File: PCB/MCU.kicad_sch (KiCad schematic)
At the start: 29 parts, among them J1 SWD, SW65 USB Boot, SW66 Reset, U2 W25Q128JVS, U3 RP2040, U7 74LVC1T45, Y1 12MHz

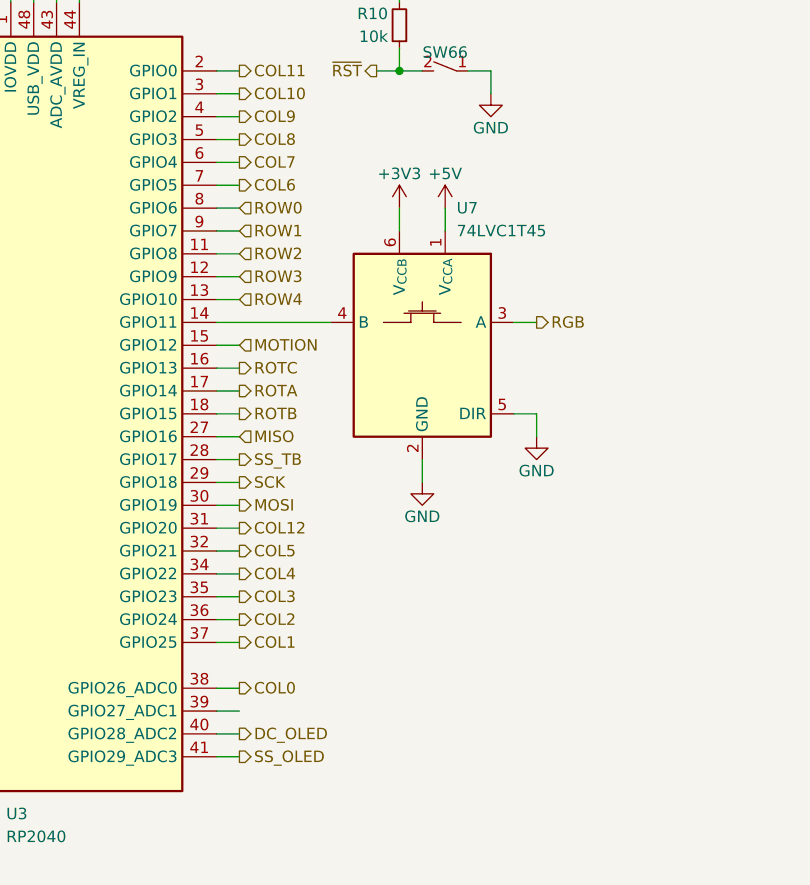
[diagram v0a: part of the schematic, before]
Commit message: Initial V2.0 update.
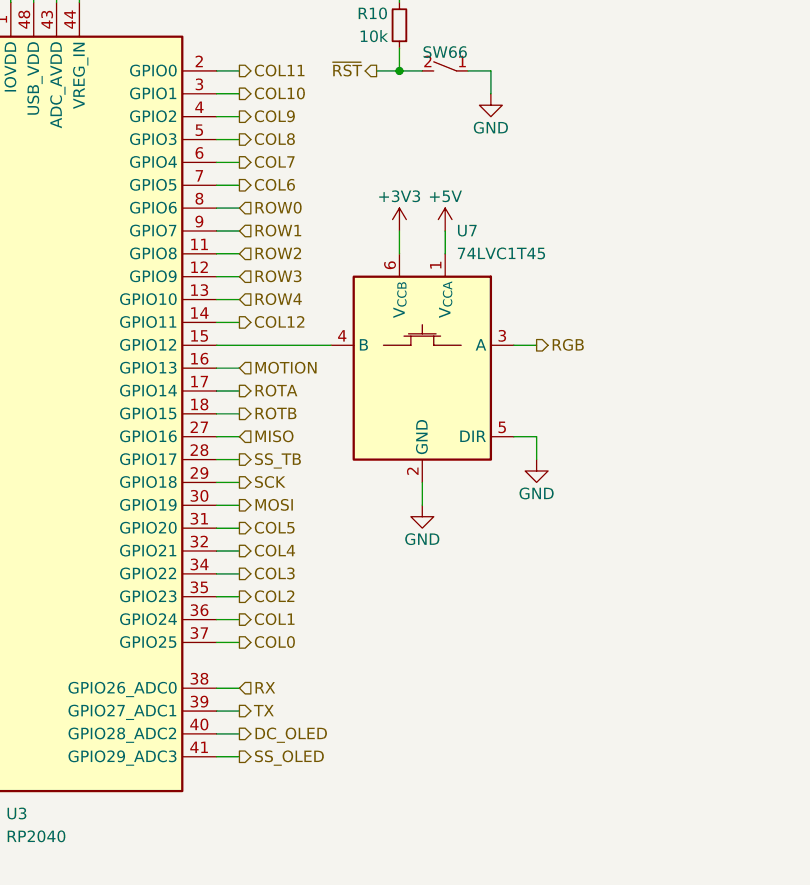
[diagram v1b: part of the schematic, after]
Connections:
- net ROTC is gone; now on net MOTION: U3.16 (GPIO13)
- net COL0: now also U3.37 (GPIO25); no longer U3.38 (GPIO26_ADC0)
- net COL1: now also U3.36 (GPIO24); no longer U3.37 (GPIO25)
- net COL12: now also U3.14 (GPIO11); no longer U3.31 (GPIO20)
- net COL2: now also U3.35 (GPIO23); no longer U3.36 (GPIO24)
- net COL3: now also U3.34 (GPIO22); no longer U3.35 (GPIO23)
- net COL4: now also U3.32 (GPIO21); no longer U3.34 (GPIO22)
- net COL5: now also U3.31 (GPIO20); no longer U3.32 (GPIO21)
- net MOTION: no longer U3.15 (GPIO12)
- net at U7.4 (B): now also U3.15 (GPIO12); no longer U3.14 (GPIO11)
- net TX: now reaches U3.39 (GPIO27_ADC1)
- new net RX: U3.38 (GPIO26_ADC0)
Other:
- moved on the sheet: U7

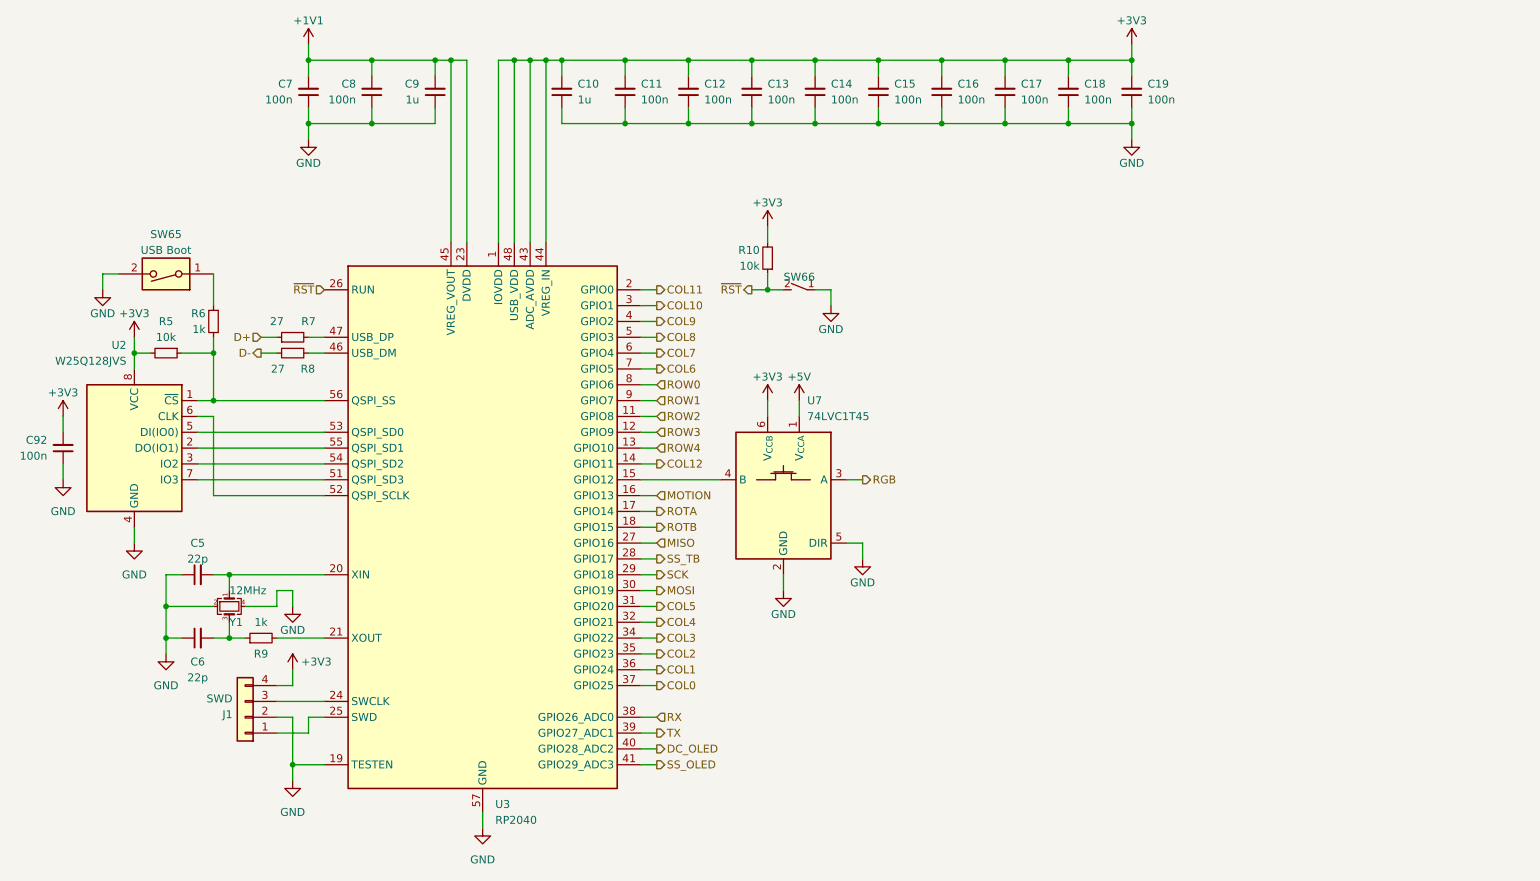
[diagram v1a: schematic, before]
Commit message: Additional changes.
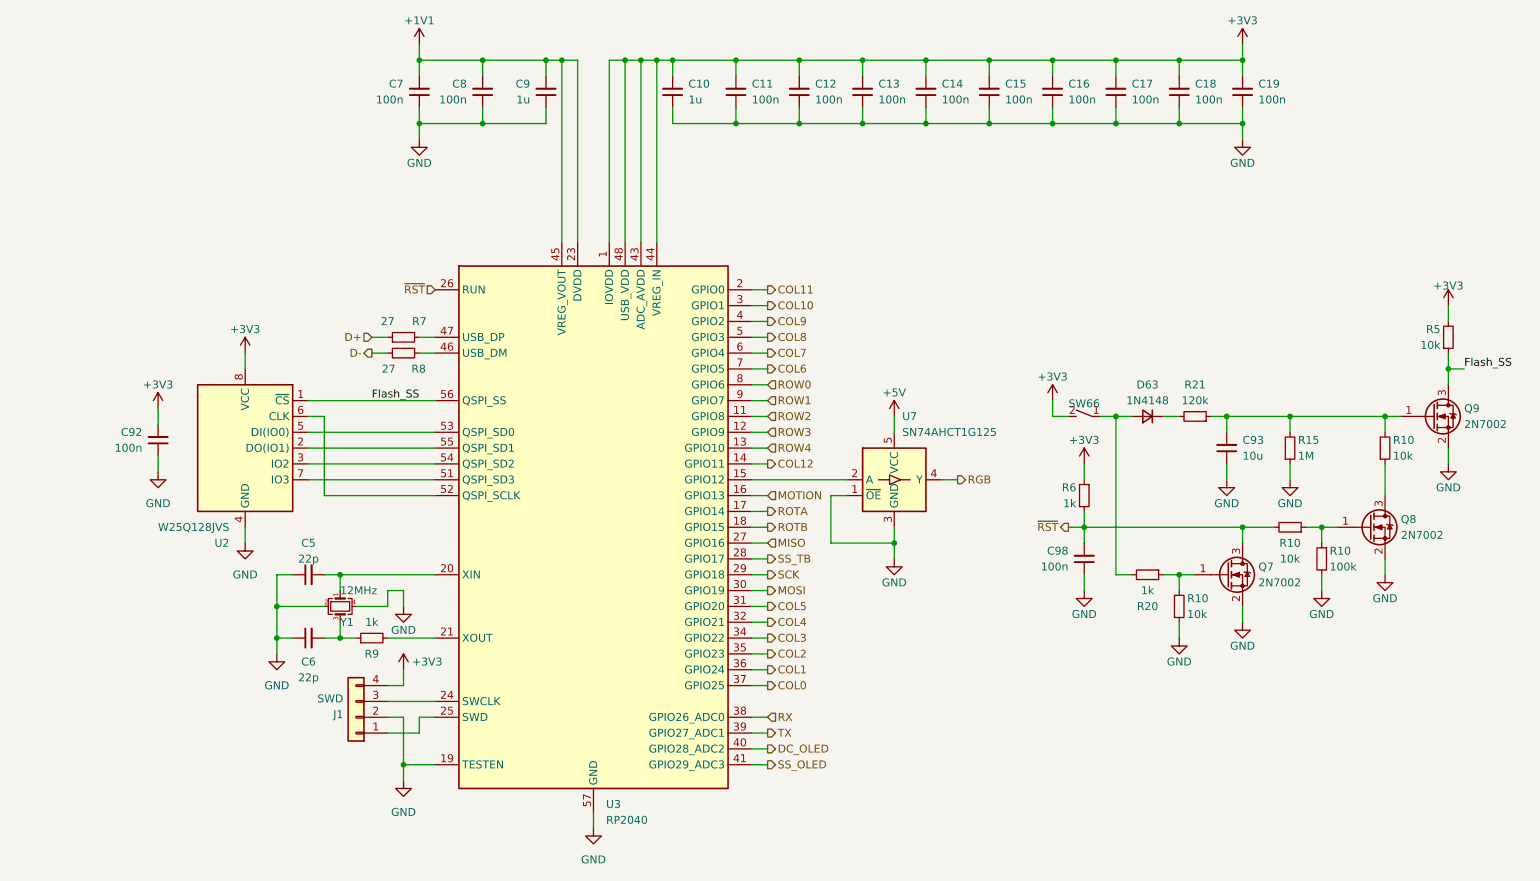
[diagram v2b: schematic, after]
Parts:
- removed R10: 10k, Resistor_SMD:R_0402_1005Metric, symbol Device:R_Small
- removed SW65: USB Boot, Button_Switch_SMD:SW_DIP_SPSTx01_Slide_6.7x4.1mm_W8.61mm_P2.54mm_LowProfile, symbol Switch:SW_DIP_x01
- removed U7: 74LVC1T45, Package_TO_SOT_SMD:SOT-363_SC-70-6, symbol Cantaloupe:74LVC1T45
- added C93: 10u, Capacitor_SMD:C_0603_1608Metric, symbol Device:C_Small
- added C98: 100n, Capacitor_SMD:C_0402_1005Metric, symbol Device:C_Small
- added D63: 1N4148, Honeydew:D_SOD-323, symbol Device:D_Small
- added Q7, Q8, Q9: 2N7002, Package_TO_SOT_SMD:SOT-23, symbol Transistor_FET:2N7002
- added R10: 100k, Resistor_SMD:R_0402_1005Metric, symbol Device:R_Small
- added R10 (x3): 10k, Resistor_SMD:R_0402_1005Metric, symbol Device:R_Small
- added R15: 1M, Resistor_SMD:R_0402_1005Metric, symbol Device:R_Small
- added R20: 1k, Resistor_SMD:R_0402_1005Metric, symbol Device:R_Small
- added R21: 120k, Resistor_SMD:R_0402_1005Metric, symbol Device:R_Small
- added U7: SN74AHCT1G125, Package_TO_SOT_SMD:SOT-23-5, symbol Honeydew:SN74AHCT1G125
- R5: now in the parts list
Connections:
- net +3V3: now also R6.1, SW66.2 (B)
- net +5V: now also U7.5 (VCC)
- net GND: now also C93.1, C98.1, Q7.2 (S), Q8.2 (S), Q9.2 (S), R10.1, R10.2, R15.1, U7.1 (~{OE}), U7.3 (GND); no longer SW66.1 (A)
- net RGB: now also U7.4 (Y)
- net ~{RST}: now also R6.2, C98.2, Q7.3 (D), R10.2; no longer SW66.2 (B)
- net Flash_SS: now reaches R5.1, U2.1 (~{CS}), U3.56 (QSPI_SS)
- net Flash_SS: now also Q9.3 (D); no longer R6.2
- net at U3.15 (GPIO12): now also U7.2 (A)
- new net: Q7.1 (G), R10.2, R20.1
- new net: Q8.1 (G), R10.1, R10.1
- new net: C93.2, Q9.1 (G), R10.2, R15.2, R21.1
- new net: Q8.3 (D), R10.1
- new net: D63.2 (A), R20.2, SW66.1 (A)
- new net: D63.1 (K), R21.2
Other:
- moved on the sheet: C10, C11, C12, C13, C14, C15, C16, C17, C18, C19, C5, C6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
